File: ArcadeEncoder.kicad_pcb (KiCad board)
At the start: 2 copper layers, 59 x 46 mm, 8 parts, among them J1 DB15_Male, J2 DB9_Male, U1 ProMicro

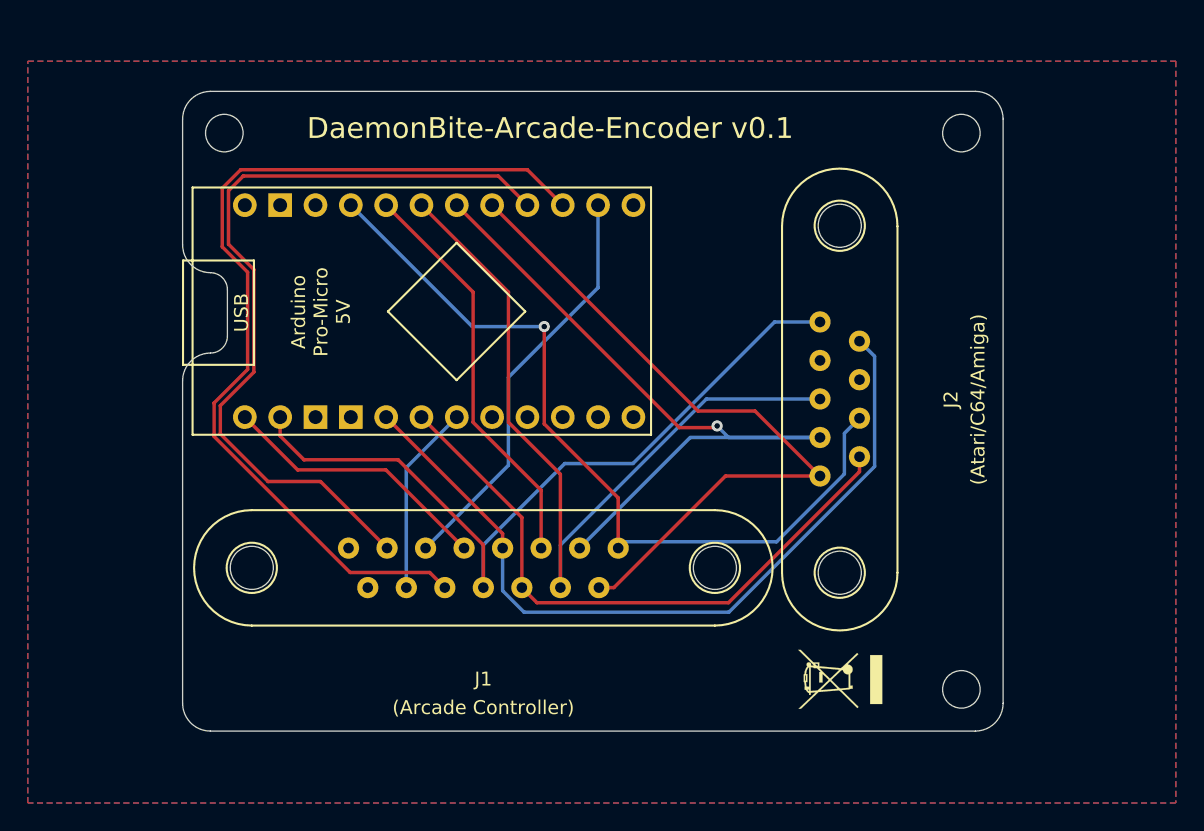
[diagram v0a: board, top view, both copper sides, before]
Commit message: v0.2
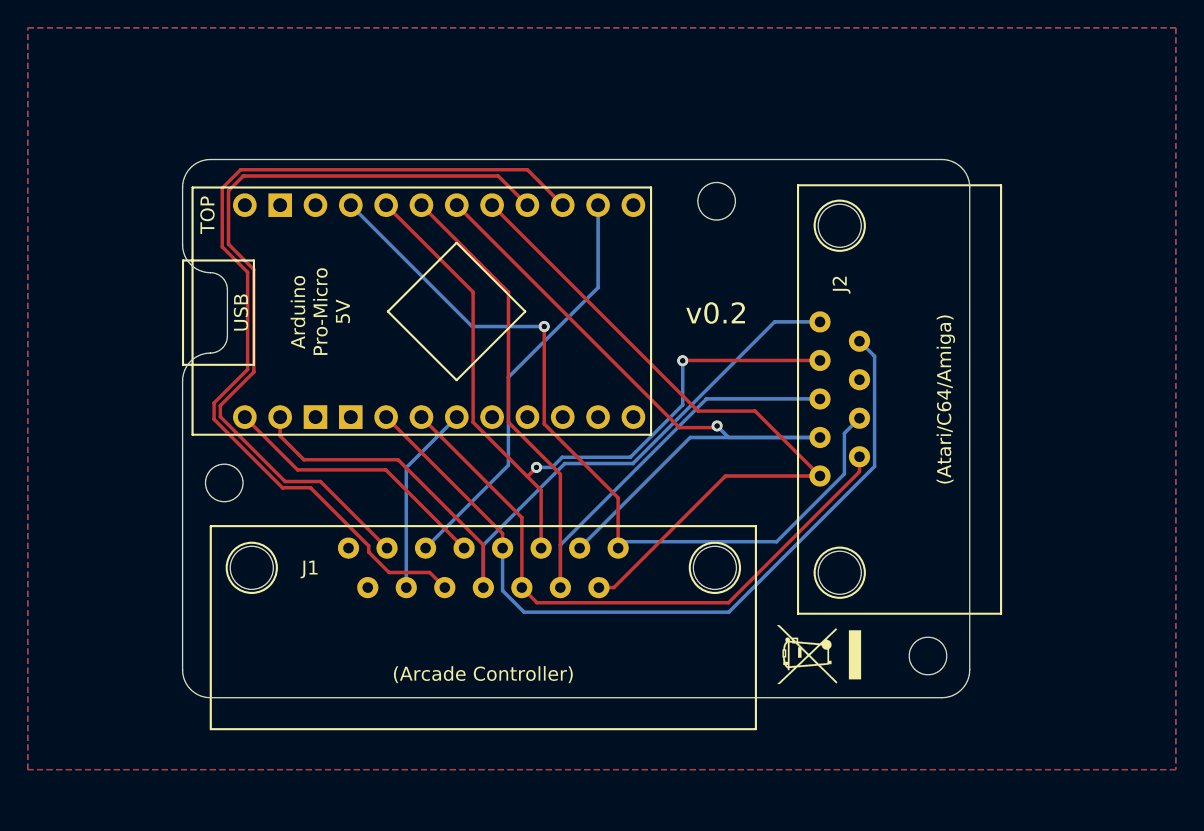
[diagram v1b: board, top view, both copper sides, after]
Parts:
- moved REF** 58.7 mm to (117.0, 67.2)
- moved REF** 35.7 mm to (152.4, 46.9)
- moved REF** 3.39 mm to (167.6, 79.6)
- moved REF** 2.34 mm to (159.8, 79.5)
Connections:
- J2 pad 4: Net-(J2-Pad4) -> RIGHT
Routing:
- net RIGHT: track 29.3 -> 55.7 mm, vias 0 -> 2
- net B6: track 57.4 -> 56.7 mm
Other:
- board size 59 x 46 mm -> 56.6 x 38.7 mm
- board text added: "TOP"
- board text added: "https://github.com/klein0r/pcb-arcade-encoder"
- board text added: "v0.2"
- board text removed: "DaemonBite-Arcade-Encoder v0.1"
